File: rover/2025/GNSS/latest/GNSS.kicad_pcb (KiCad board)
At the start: 4 copper layers, 50 x 50 mm, 39 parts, among them J1 Eth-Horiz, J2 Eth-Horiz, J4 JST6_Pin, J5 USB_C_USB4145-GCT, SW1 TS09-63-25-WT-160-SMT-TR, SW2 TS09-63-25-WT-160-SMT-TR, U1 SN65HVD232, U2 ESP32-S3-WROVER, U4 LDO-TLV74033PDBVR, U5 TVS, U6 DC_DC-AP64501

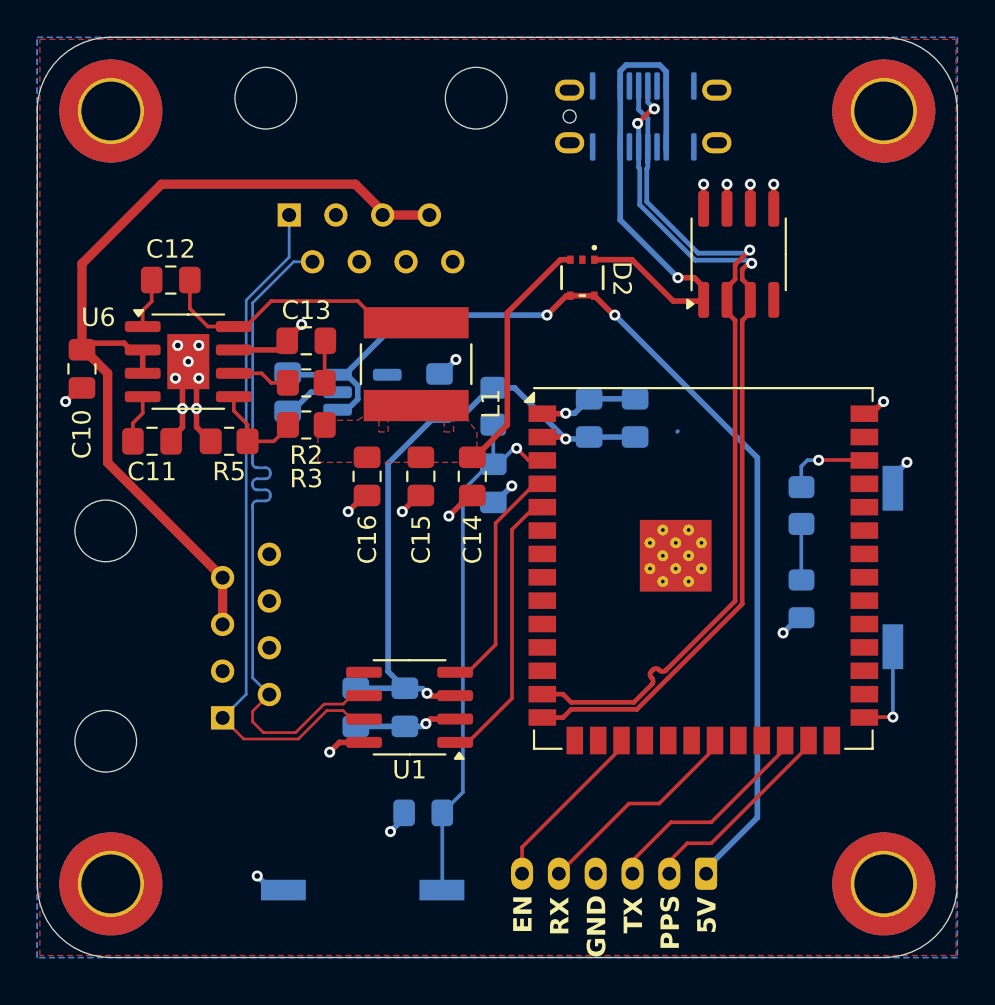
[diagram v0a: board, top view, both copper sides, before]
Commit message: gnss update
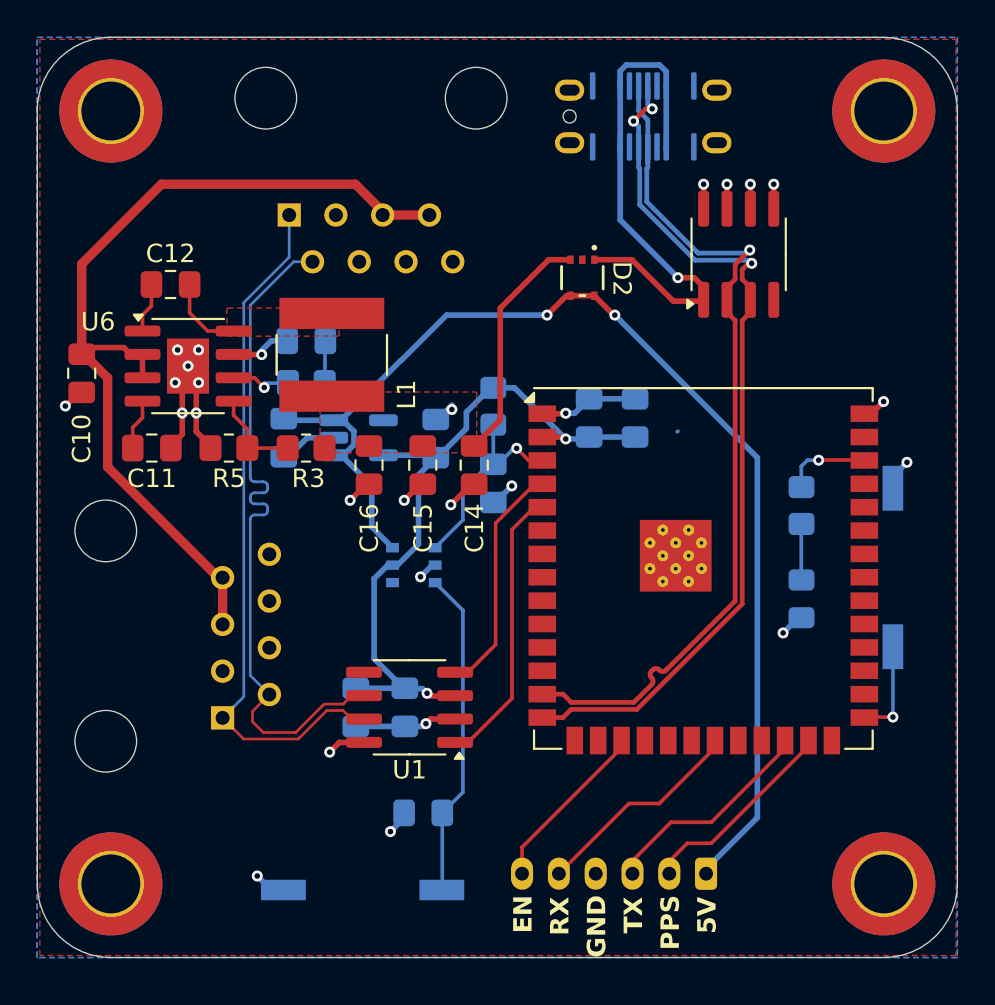
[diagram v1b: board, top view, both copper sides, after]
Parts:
- added U3: Volt_check-NCV308, Package_SO:TSOP-6_1.65x3.05mm_P0.95mm, B.Cu at (148.5, 98.7)
- C13, R2: moved to B.Cu
- moved L1 4.61 mm to (144.0, 87.2)
- moved C5 2.48 mm to (149.7, 91.8)
- moved U4 2.48 mm to (145.5, 91.8)
- moved C6 2.48 mm to (141.4, 91.8)
- moved R3 1.26 mm to (142.6, 92.3)
- moved C14 0.62 mm to (151.7, 93.2)
- moved C15 0.62 mm to (148.9, 93.2)
- moved C16 0.62 mm to (146.0, 93.2)
- moved C11 0.37 mm to (134.2, 92.3)
- moved R5 0.37 mm to (138.4, 92.3)
- moved C10 0.24 mm to (130.4, 88.3)
- moved C12 0.24 mm to (135.2, 83.4)
- moved U6 0.24 mm to (136.2, 87.9)
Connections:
- C1 pad 1: EN_ESP -> EN_SW
- SW1 pad 1: EN_ESP -> EN_SW
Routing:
- net EN_ESP: track 29.9 -> 11.4 mm
- net EN_SW: track 0.00 -> 17.8 mm
- net Net-(U6-SW): track 15.3 -> 4.99 mm
- net +5V: track 58.2 -> 64.6 mm
- net +5V_ETH: track 19.6 -> 13.2 mm
- net Net-(U6-COMB): track 3.15 -> 3.53 mm, vias 0 -> 1
- net GND: vias 26 -> 27
- added copper zone on F.Cu, net Net-(U6-SW)
